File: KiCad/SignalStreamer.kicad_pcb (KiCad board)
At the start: 2 copper layers, 100.3 x 59.1 mm, 48 parts, among them J105 Conn_01x02, T101 Coupled_Inductors_2

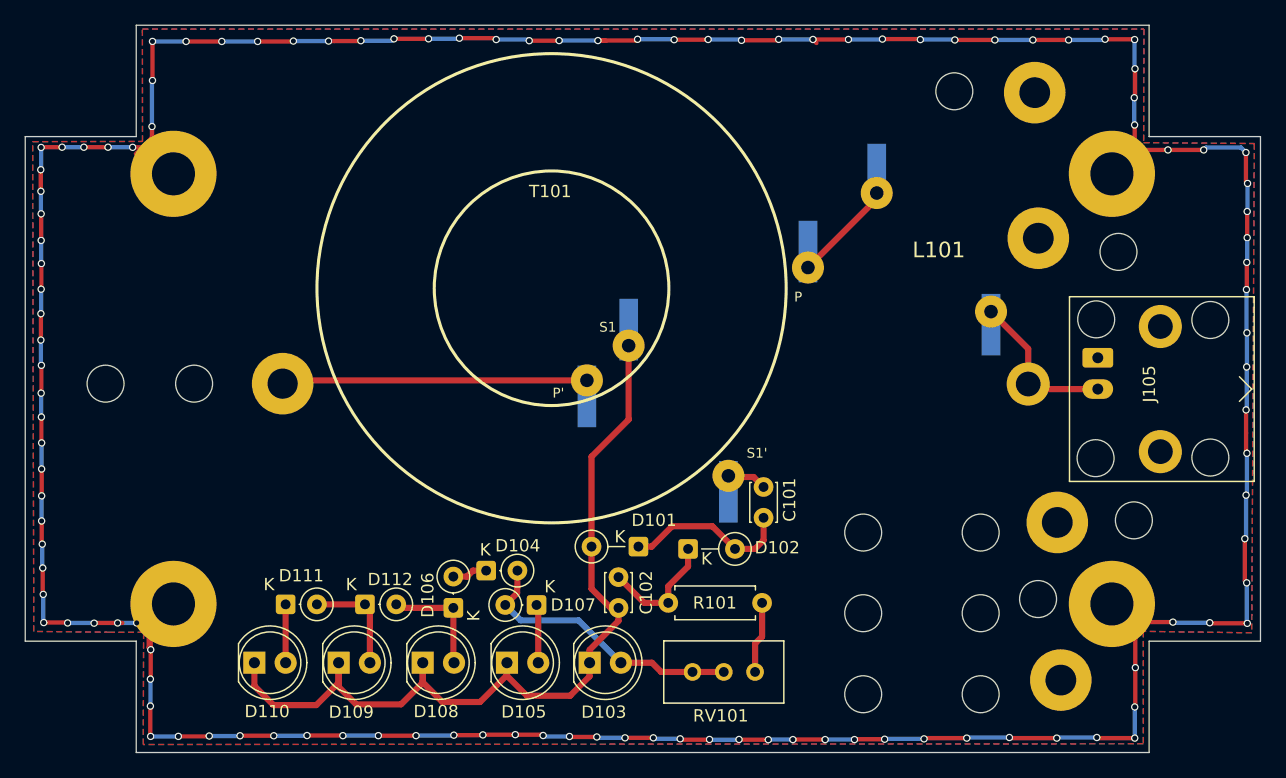
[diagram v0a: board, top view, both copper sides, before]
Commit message: Ver X1.0
Copied latest changes from backup project
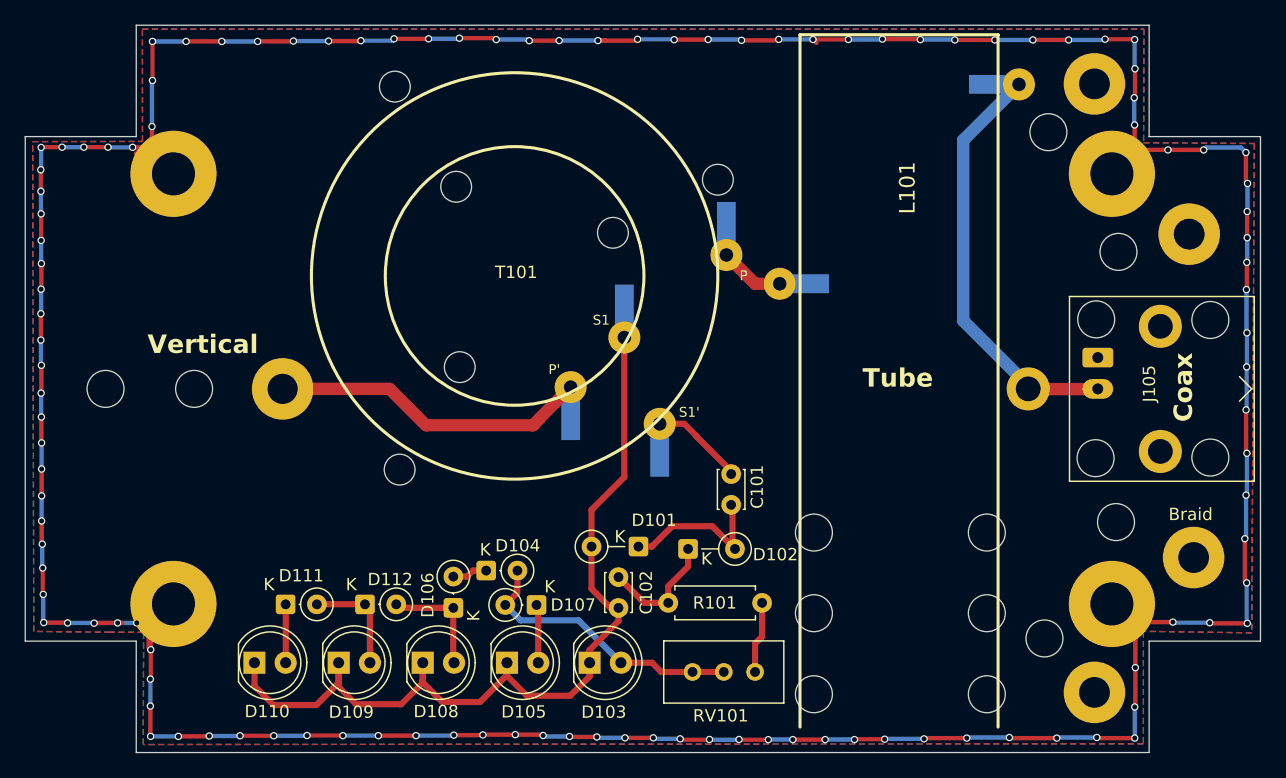
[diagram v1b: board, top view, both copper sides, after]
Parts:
- added REF**: MountingHole_2.5mm, MountingHole:MountingHole_2.5mm, F.Cu at (75.2, 86.3)
- added REF**: MountingHole_2.5mm, MountingHole:MountingHole_2.5mm, F.Cu at (96.1, 71.0)
- added REF**: MountingHole_2.5mm, MountingHole:MountingHole_2.5mm, F.Cu at (87.6, 75.4)
- added REF**: MountingHole_2.5mm, MountingHole:MountingHole_2.5mm, F.Cu at (69.9, 63.5)
- added REF**: MountingHole_2.5mm, MountingHole:MountingHole_2.5mm, F.Cu at (74.9, 71.6)
- added REF**: MountingHole_2.5mm, MountingHole:MountingHole_2.5mm, F.Cu at (70.3, 94.6)
- T101: footprint Inductor_THT:Core_150A_2_windings_Horiz_TH -> Inductor_THT:Core_T130_2_windings_Horiz_TH
- moved L101 19.5 mm to (119.0, 63.3), turned to -90 degrees
- moved L101 18.6 mm to (120.6, 63.3), turned to -90 degrees
- moved REF** 12.3 mm to (134.4, 75.5)
- moved REF** 11.4 mm to (134.8, 101.7)
- moved L101 10.9 mm to (102.7, 79.5), turned to -90 degrees
- moved L101 10.8 mm to (101.2, 79.5), turned to -90 degrees
- moved ? 8.33 mm to (123.0, 67.2)
- moved REF** 4.90 mm to (126.7, 63.3)
- moved ? 4.00 mm to (103.9, 106.2)
- moved ? 4.00 mm to (103.9, 112.8)
- moved REF** 4.00 mm to (103.9, 99.7)
- moved ? 3.24 mm to (122.7, 108.3)
- moved T101 3.16 mm to (79.6, 78.9)
- moved REF** 2.91 mm to (126.7, 112.7)
- moved C101 2.83 mm to (97.2, 97.5)
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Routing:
- net Net-(J105-Pin_1): track 13.0 -> 34.3 mm
- net Net-(T101-IN+): track 3.23 -> 7.65 mm
- net Net-(T101-OUT1B): track 8.37 -> 5.29 mm
- net Net-(AE101-A): track 24.8 -> 27.3 mm
- net Net-(D101-K): track 13.7 -> 13.0 mm
- net Net-(D101-A): track 74.0 -> 74.5 mm
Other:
- board text added: "*"
- board text added: "Braid"
- board text added: "Coax"
- board text added: "Counterpoise Elements*"
- board text added: "SignalStreamer Ver 1.0 1 Jan 2026"
- board text added: "Tube"
- board text added: "Vertical"
